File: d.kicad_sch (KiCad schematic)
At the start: 114 parts, among them J1 Conn_01x18_Pin, J2 Conn_01x03_Pin, K1 Fujitsu_FTR-LYCA005x, K2 Fujitsu_FTR-LYCA005x, K3 Fujitsu_FTR-LYCA005x, K4 Fujitsu_FTR-LYCA005x, K5 Fujitsu_FTR-LYCA005x, K6 Fujitsu_FTR-LYCA005x, K7 Fujitsu_FTR-LYCA005x, K9 Fujitsu_FTR-LYCA005x, Q1 BC547, Q2 BC547, Q3 BC547, Q4 BC547, Q5 BC547, Q6 BC547, Q7 BC547, Q8 BC547, U1 VIPer22AS, U10 GP2S700HCP, U2 GP2S700HCP, U3 TL431D, U4 VIPer22AS, U5 GP2S700HCP, U6 TL431D, U7 ESP32-WROOM-32, U8 GP2S700HCP, U9 GP2S700HCP

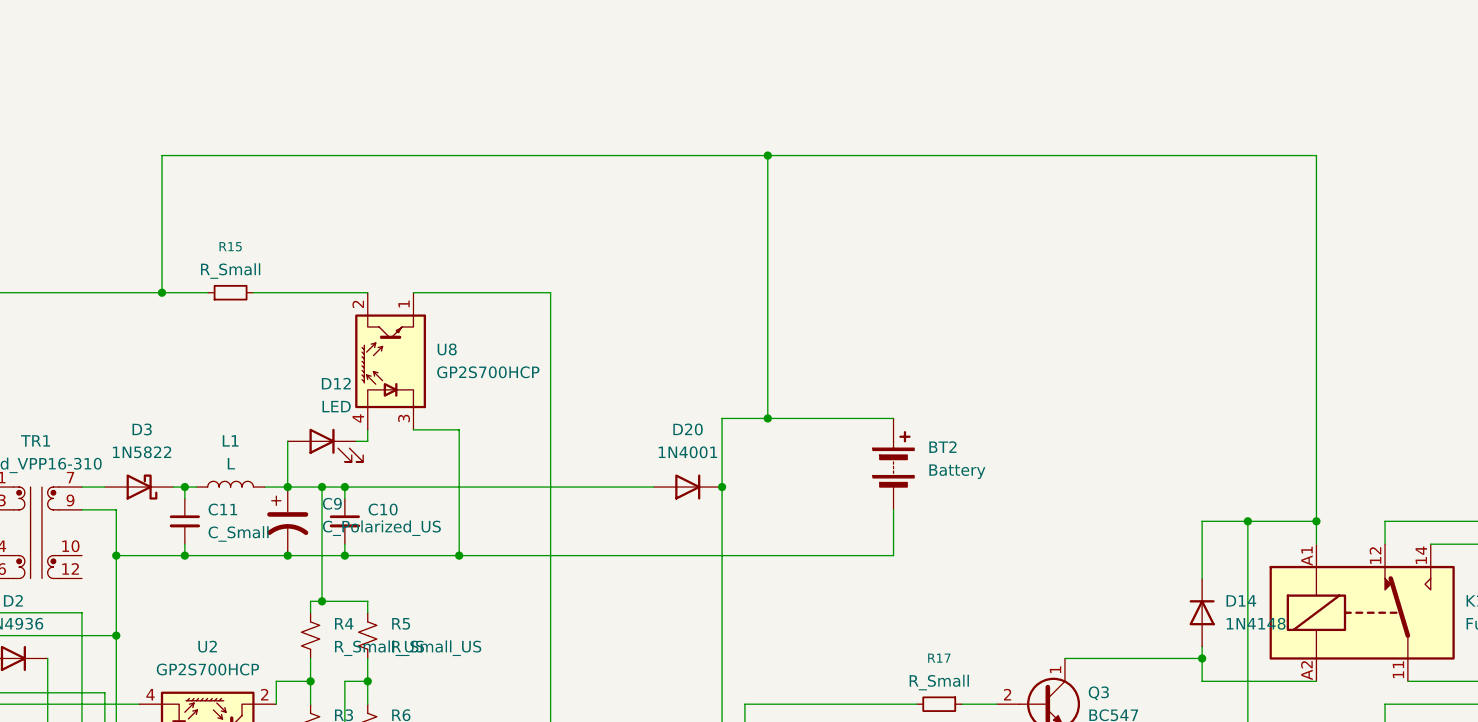
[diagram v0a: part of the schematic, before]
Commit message: Add files via upload
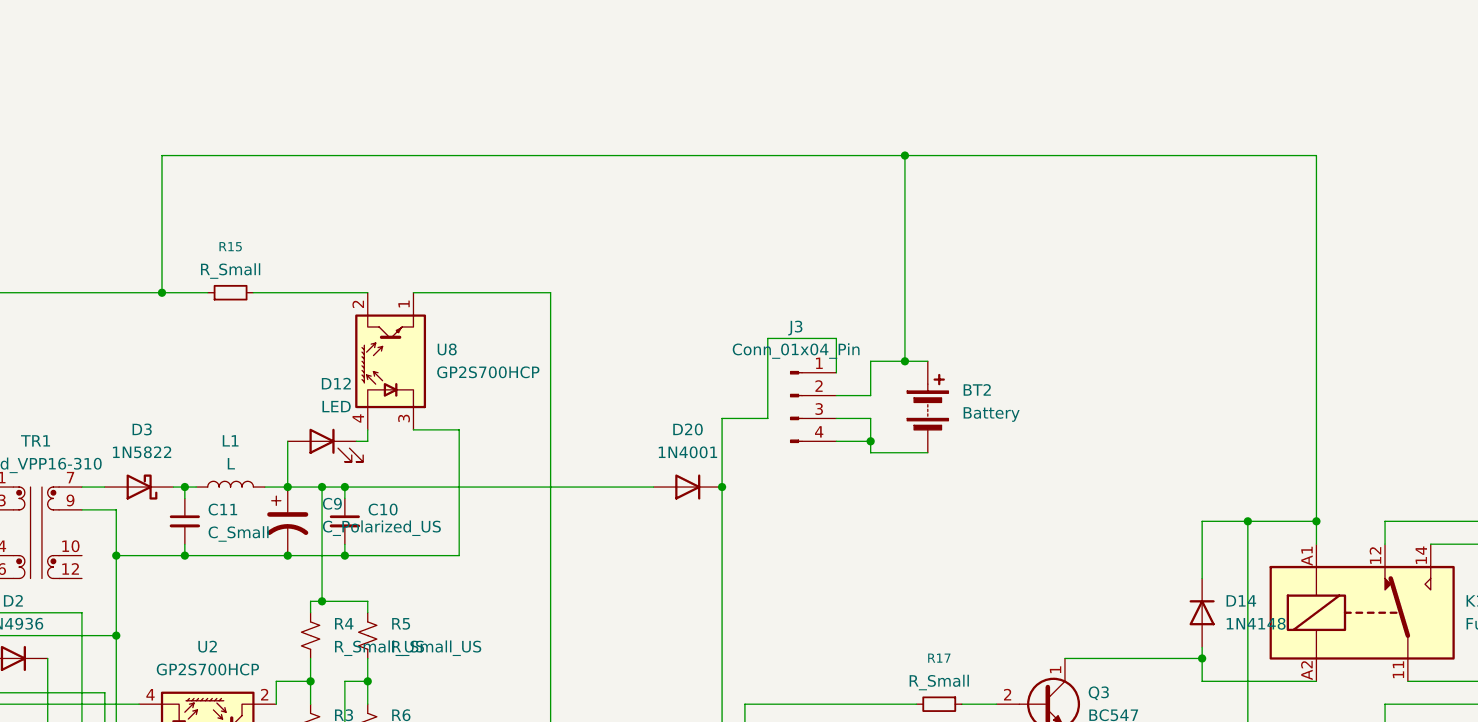
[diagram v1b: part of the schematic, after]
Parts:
- added J3: Conn_01x04_Pin, Connector_PinHeader_2.00mm:PinHeader_1x04_P2.00mm_Vertical, symbol Connector:Conn_01x04_Pin
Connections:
- net Earth: no longer BT2.2 (-)
- net VCC: now also J3.2 (Pin_2); no longer D20.1 (K), D21.1 (K), D22.1 (K)
- new net: D20.1 (K), D21.1 (K), D22.1 (K), J3.1 (Pin_1)
- new net: BT2.2 (-), J3.3 (Pin_3), J3.4 (Pin_4)
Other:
- moved on the sheet: BT2
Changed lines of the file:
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@@
 	)
 	(junction
-		(at 269.24 92.71)
-		(diameter 0)
-		(color 0 0 0 0)
-	)
-	(junction
 		(at 77.47 104.14)
 		(diameter 0)
@@
 	)
 	(junction
-		(at 303.53 48.26)
-		(diameter 0)
-		(color 0 0 0 0)
-	)
-	(junction
 		(at 256.54 92.71)
 		(diameter 0)
@@
 	)
 	(junction
+		(at 318.77 71.12)
+		(diameter 0)
+		(color 0 0 0 0)
+	)
+	(junction
 		(at 146.05 170.18)
 		(diameter 0)
@@
 	)
 	(junction
-		(at 217.17 113.03)
+		(at 318.77 48.26)
 		(diameter 0)
 		(color 0 0 0 0)
 	)
 	(junction
-		(at 247.65 166.37)
+		(at 217.17 113.03)
 		(diameter 0)
 		(color 0 0 0 0)
 	)
 	(junction
-		(at 236.22 63.5)
+		(at 247.65 166.37)
 		(diameter 0)
 		(color 0 0 0 0)
 	)
 	(junction
-		(at 303.53 77.47)
+		(at 236.22 63.5)
 		(diameter 0)
 		(color 0 0 0 0)
@@
 	)
 	(junction
+		(at 314.96 80.01)
+		(diameter 0)
+		(color 0 0 0 0)
+	)
+	(junction
 		(at 205.74 91.44)
 		(diameter 0)
@@
 	(wire
 		(pts
-			(xy 214.63 120.65) (xy 214.63 105.41)
+			(xy 303.53 68.58) (xy 311.15 68.58)
 		)
 		(stroke
@@
 	(wire
 		(pts
-			(xy 207.01 168.91) (xy 207.01 180.34)
+			(xy 214.63 120.65) (xy 214.63 105.41)
 		)
 		(stroke
@@
 	(wire
 		(pts
-			(xy 175.26 93.98) (xy 175.26 92.71)
+			(xy 207.01 168.91) (xy 207.01 180.34)
 		)
 		(stroke
@@
 	(wire
 		(pts
-			(xy 252.73 104.14) (xy 252.73 106.68)
+			(xy 175.26 93.98) (xy 175.26 92.71)
 		)
 		(stroke
@@
 	(wire
 		(pts
-			(xy 217.17 92.71) (xy 214.63 92.71)
+			(xy 252.73 104.14) (xy 252.73 106.68)
 		)
 		(stroke
@@
 	(wire
 		(pts
-			(xy 161.29 181.61) (xy 167.64 181.61)
+			(xy 217.17 92.71) (xy 214.63 92.71)
 		)
 		(stroke
@@
 	(wire
 		(pts
-			(xy 101.6 101.6) (xy 123.19 101.6)
+			(xy 161.29 181.61) (xy 167.64 181.61)
 		)
 		(stroke
@@
 	(wire
 		(pts
-			(xy 317.5 77.47) (xy 303.53 77.47)
+			(xy 101.6 101.6) (xy 123.19 101.6)
 		)
 		(stroke
@@
 	(wire
 		(pts
+			(xy 314.96 81.28) (xy 321.31 81.28)
+		)
+		(stroke
+			(width 0)
+			(type default)
+		)
+	)
+	(wire
+		(pts
 			(xy 110.49 91.44) (xy 106.68 91.44)
 		)
@@
 	(wire
 		(pts
+			(xy 303.53 77.47) (xy 303.53 68.58)
+		)
+		(stroke
+			(width 0)
+			(type default)
+		)
+	)
+	(wire
+		(pts
 			(xy 391.16 144.78) (xy 402.59 144.78)
 		)
@@
 	(wire
 		(pts
+			(xy 311.15 68.58) (xy 311.15 72.39)
+		)
+		(stroke
+			(width 0)
+			(type default)
+		)
+	)
+	(wire
+		(pts
 			(xy 208.28 85.09) (xy 208.28 83.82)
 		)
@@
 	(wire
 		(pts
-			(xy 303.53 48.26) (xy 303.53 77.47)
-		)
-		(stroke
-			(width 0)
-			(type default)
-		)
-	)
-	(wire
-		(pts
 			(xy 49.53 133.35) (xy 91.44 133.35)
 		)
@@
 	(wire
 		(pts
-			(xy 236.22 48.26) (xy 303.53 48.26)
+			(xy 318.77 48.26) (xy 318.77 71.12)
+		)
+		(stroke
+			(width 0)
+			(type default)
+		)
+	)
+	(wire
+		(pts
+			(xy 236.22 48.26) (xy 318.77 48.26)
 		)
 		(stroke
@@
 	(wire
 		(pts
-			(xy 317.5 87.63) (xy 317.5 92.71)
-		)
-		(stroke
-			(width 0)
-			(type default)
-		)
-	)
-	(wire
-		(pts
 			(xy 127 88.9) (xy 127 90.17)
 		)
@@
 	(wire
 		(pts
+			(xy 311.15 74.93) (xy 314.96 74.93)
+		)
+		(stroke
+			(width 0)
+			(type default)
+		)
+	)
+	(wire
+		(pts
 			(xy 402.59 157.48) (xy 372.11 157.48)
 		)
@@
 	(wire
 		(pts
-			(xy 196.85 172.72) (xy 199.39 172.72)
+			(xy 311.15 80.01) (xy 314.96 80.01)
 		)
 		(stroke
@@
 	(wire
 		(pts
-			(xy 110.49 68.58) (xy 110.49 81.28)
+			(xy 196.85 172.72) (xy 199.39 172.72)
 		)
 		(stroke
@@
 	(wire
 		(pts
-			(xy 269.24 92.71) (xy 317.5 92.71)
+			(xy 110.49 68.58) (xy 110.49 81.28)
 		)
 		(stroke
@@
 	(wire
 		(pts
+			(xy 318.77 71.12) (xy 321.31 71.12)
+		)
+		(stroke
+			(width 0)
+			(type default)
+		)
+	)
+	(wire
+		(pts
 			(xy 142.24 177.8) (xy 137.16 177.8)
 		)
@@
 	(wire
 		(pts
+			(xy 314.96 71.12) (xy 318.77 71.12)
+		)
+		(stroke
+			(width 0)
+			(type default)
+		)
+	)
+	(wire
+		(pts
 			(xy 256.54 86.36) (xy 256.54 85.09)
 		)
@@
 	(wire
 		(pts
+			(xy 314.96 74.93) (xy 314.96 71.12)
+		)
+		(stroke
+			(width 0)
+			(type default)
+		)
+	)
+	(wire
+		(pts
 			(xy 148.59 96.52) (xy 143.51 96.52)
 		)
@@
 	(wire
 		(pts
+			(xy 318.77 48.26) (xy 364.49 48.26)
+		)
+		(stroke
+			(width 0)
+			(type default)
+		)
+	)
+	(wire
+		(pts
 			(xy 293.37 262.89) (xy 83.82 262.89)
 		)
@@
 	(wire
 		(pts
+			(xy 311.15 77.47) (xy 314.96 77.47)
+		)
+		(stroke
+			(width 0)
+			(type default)
+		)
+	)
+	(wire
+		(pts
+			(xy 314.96 77.47) (xy 314.96 80.01)
+		)
+		(stroke
+			(width 0)
+			(type default)
+		)
+	)
+	(wire
+		(pts
+			(xy 314.96 80.01) (xy 314.96 81.28)
+		)
+		(stroke
+			(width 0)
+			(type default)
+		)
+	)
+	(wire
+		(pts
 			(xy 356.87 212.09) (xy 351.79 212.09)
 		)
@@
 	(wire
 		(pts
-			(xy 303.53 48.26) (xy 364.49 48.26)
-		)
-		(stroke
-			(width 0)
-			(type default)
-		)
-	)
-	(wire
-		(pts
 			(xy 220.98 209.55) (xy 219.71 209.55)
 		)
@@
 	(symbol
 		(lib_id "Device:Battery")
-		(at 317.5 82.55 0)
+		(at 321.31 76.2 0)
 		(unit 1)
 		(exclude_from_sim no)
@@
 		(fields_autoplaced yes)
 		(property "Reference" "BT2"
-			(at 321.31 80.7084 0)
+			(at 325.12 74.3584 0)
 			(effects
 				(font
@@
 		)
 		(property "Value" "Battery"
-			(at 321.31 83.2484 0)
+			(at 325.12 76.8984 0)
 			(effects
 				(font
@@
 		)
 		(property "Footprint" "Battery:BatteryHolder_MYOUNG_BS-07-A1BJ001_CR2032"
-			(at 317.5 81.026 90)
+			(at 321.31 74.676 90)
 			(effects
 				(font
@@
 		)
 		(property "Datasheet" "~"
-			(at 317.5 81.026 90)
+			(at 321.31 74.676 90)
 			(effects
 				(font
@@
 		)
 		(property "Description" "Multiple-cell battery"
-			(at 317.5 82.55 0)
+			(at 321.31 76.2 0)
 			(effects
 				(font
@@
 					(unit 1)
 				)
+			)
+		)
+	)
+	(symbol
+		(lib_id "Connector:Conn_01x04_Pin")
+		(at 306.07 74.93 0)
+		(unit 1)
+		(exclude_from_sim no)
+		(in_bom yes)
+		(on_board yes)
+		(dnp no)
+		(fields_autoplaced yes)
+		(property "Reference" "J3"
+			(at 306.705 67.31 0)
+			(effects
+				(font
+					(size 1.27 1.27)
+				)
+			)
+		)
+		(property "Value" "Conn_01x04_Pin"
+			(at 306.705 69.85 0)
+			(effects
+				(font
+					(size 1.27 1.27)
+				)
+			)
+		)
+		(property "Footprint" "Connector_PinHeader_2.00mm:PinHeader_1x04_P2.00mm_Vertical"
+			(at 306.07 74.93 0)
+			(effects
+				(font
+					(size 1.27 1.27)
+				)
+				(hide yes)
+			)
+		)
+		(property "Datasheet" "~"
+			(at 306.07 74.93 0)
+			(effects
+				(font
+					(size 1.27 1.27)
+				)
+				(hide yes)
+			)
+		)
+		(property "Description" "Generic connector, single row, 01x04, script generated"
+			(at 306.07 74.93 0)
+			(effects
+				(font
+					(size 1.27 1.27)
+				)
+				(hide yes)
+			)
+		)
+		(pin "3"
+		)
+		(pin "1"
+		)
+		(pin "2"
+		)
+		(pin "4"
+		)
+		(instances
+			(project ""
+				(path "/f2f788d2-6a74-400b-8c1e-3985a57e88b9"
+					(reference "J3")
+					(unit 1)
+				)
